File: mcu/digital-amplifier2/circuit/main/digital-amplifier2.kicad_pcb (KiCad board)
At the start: 2 copper layers, 94.5 x 100 mm, 166 parts, among them J1 I2C_oled, J10 Audio outA, J11 Audio outB, J12 Audio outC, J13 Audio outD, J2 encoder, J3 USB_C_Receptacle, J4 Conn_ARM_JTAG_SWD_20, J5 Barrel_Jack_Switch, J6 Conn_02x10_Odd_Even, J7 Conn_Coaxial, Q1 S8550, Q2 S8050, Q3 S8550, Q4 Q_NMOS_GDS, U1 DLT11H0, U12 TAS6424QDKQRQ1, U13 SJR-BTM331, U2 STM32F446RETx, U3 TPS54360DDA, U4 AMS1117-3.3, U5 LT3045xMSE-1, Y1 5032 8m

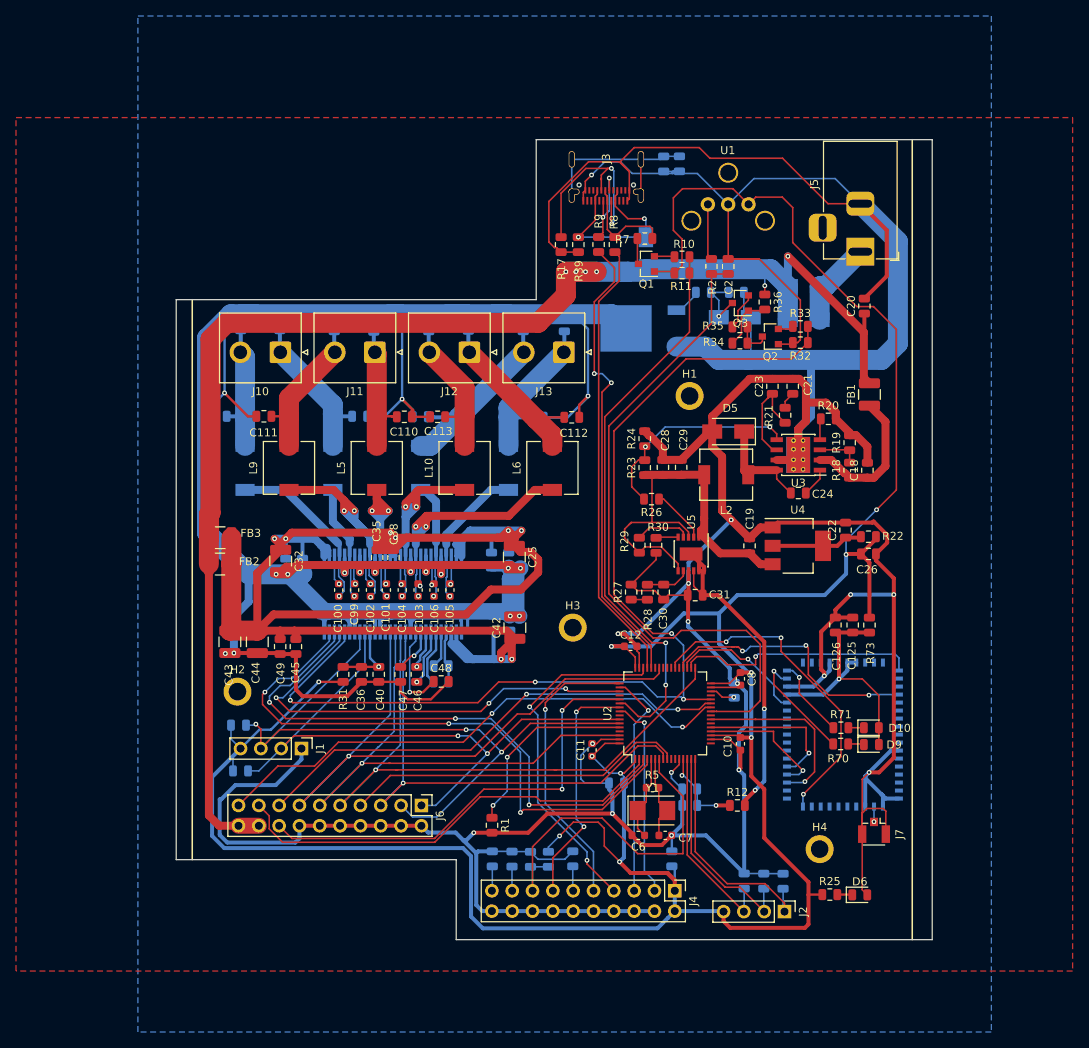
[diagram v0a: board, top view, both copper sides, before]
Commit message: headphone
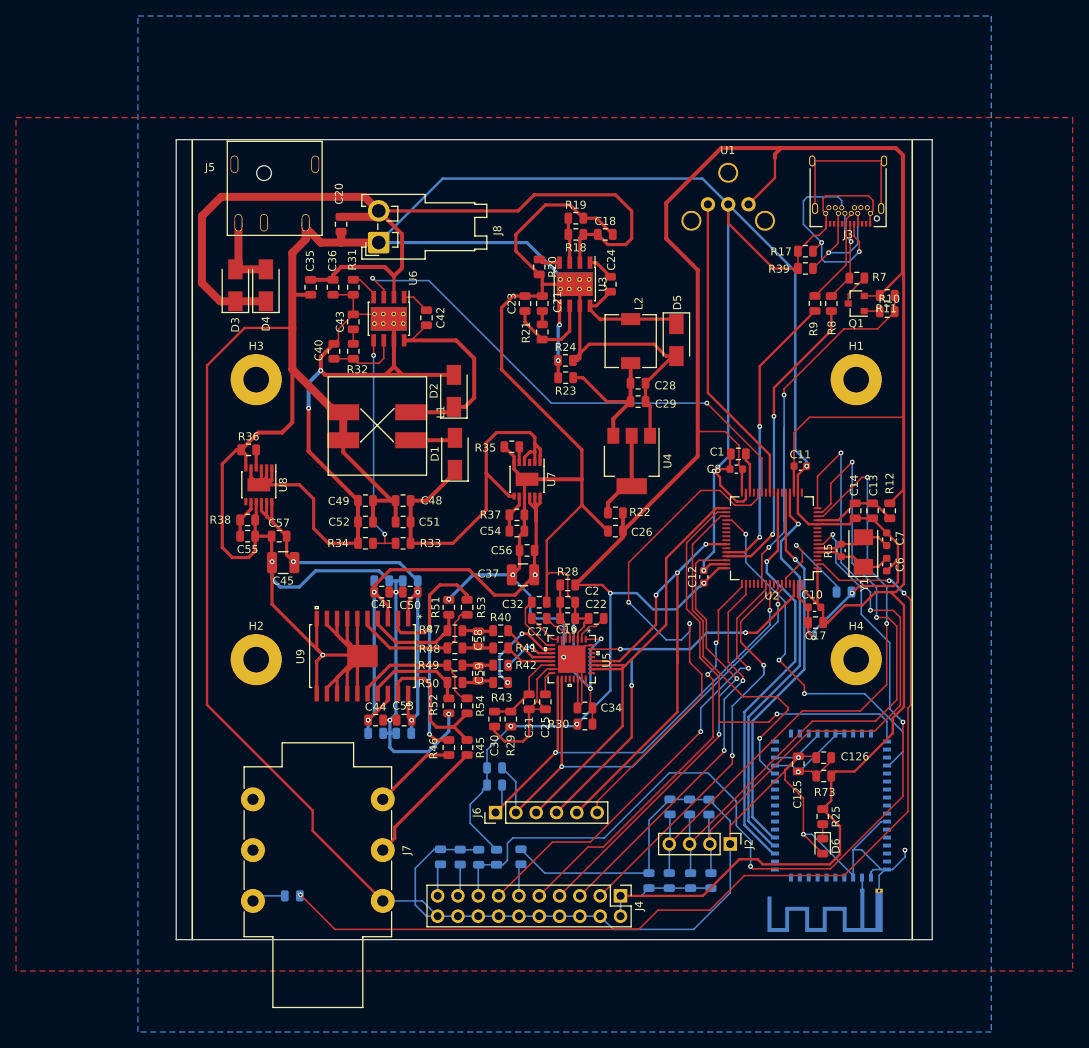
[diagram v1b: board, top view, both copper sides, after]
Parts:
- removed C100, C101, C102, C103, C104, C105, C106, C99: 1uf, Capacitor_SMD:C_0603_1608Metric
- removed C108, C109, C110, C111, C112, C113, C114, C115, C87, C88: 1uf, Capacitor_SMD:C_0805_2012Metric
- removed C117, C118, C119, C120, C121, C122, C123, C124: 1nf, Capacitor_SMD:C_0805_2012Metric
- removed C9: 1nF/1KV, Capacitor_SMD:C_0805_2012Metric
- removed D10, D9: LED, LED_SMD:LED_0805_2012Metric
- removed FB1, FB2, FB3: 300 ohm @100MHz 3.1A, Inductor_SMD:L_1210_3225Metric
- removed J1: I2C_oled, Connector_PinHeader_2.54mm:PinHeader_1x04_P2.54mm_Vertical
- removed J10: Audio outA, Connector_JST:JST_NV_B02P-NV_1x02_P5.00mm_Vertical
- removed J11: Audio outB, Connector_JST:JST_NV_B02P-NV_1x02_P5.00mm_Vertical
- removed J12: Audio outC, Connector_JST:JST_NV_B02P-NV_1x02_P5.00mm_Vertical
- removed J13: Audio outD, Connector_JST:JST_NV_B02P-NV_1x02_P5.00mm_Vertical
- removed L10, L11, L4, L5, L6, L7, L8, L9: 3.3uh, Inductor_SMD:L_6.3x6.3_H3
- removed Q2: S8050, Package_TO_SOT_SMD:SOT-23
- removed Q3: S8550, Package_TO_SOT_SMD:SOT-23
- removed Q4: Q_NMOS_GDS, Package_TO_SOT_SMD:TO-252-2
- removed R6: 1m, Resistor_SMD:R_0805_2012Metric
- removed R70, R71: 1k, Resistor_SMD:R_0805_2012Metric
- removed U12: TAS6424QDKQRQ1, ti:TAS6424QDKQRQ1
- added AE1: Antenna_Shield, RF_Antenna:Texas_SWRA117D_2.4GHz_Left, B.Cu at (135.8, 143.9)
- added C33: 100nf, Capacitor_SMD:C_0805_2012Metric, B.Cu at (98.9, 109.9)
- added C51: 22uf, Capacitor_SMD:C_0805_2012Metric, F.Cu at (78.4, 97.8)
- added C52: 22uf, Capacitor_SMD:C_0805_2012Metric, F.Cu at (73.7, 97.8)
- added C53: 100nf, Capacitor_SMD:C_0805_2012Metric, F.Cu at (78.5, 122.6)
- added C54: 4.7uf, Capacitor_SMD:C_0805_2012Metric, F.Cu at (92.6, 98.9)
- added C55: 4.7uf, Capacitor_SMD:C_0805_2012Metric, F.Cu at (58.9, 99.6)
- added C56: 10uf, Capacitor_SMD:C_0805_2012Metric, F.Cu at (93.9, 101.3)
- added C57: 10uf, Capacitor_SMD:C_0805_2012Metric, F.Cu at (62.9, 99.6)
- added C58: 100pf, Capacitor_SMD:C_0805_2012Metric, F.Cu at (87.8, 112.4)
- added C59: 100pf, Capacitor_SMD:C_0805_2012Metric, F.Cu at (87.8, 116.7)
- added J8: Conn_01x02, Connector_JST:JST_VH_S2P-VH_1x02_P3.96mm_Horizontal, F.Cu at (75.3, 62.9)
- added L1: 150uh, misc:MSD1278, F.Cu at (79.4, 84.1)
- added R40: 402Ω, Resistor_SMD:R_0805_2012Metric, F.Cu at (90.6, 111.4)
- added R41: 402Ω, Resistor_SMD:R_0805_2012Metric, F.Cu at (90.6, 113.5)
- added R42: 402Ω, Resistor_SMD:R_0805_2012Metric, F.Cu at (90.6, 115.7)
- added R43: 402Ω, Resistor_SMD:R_0805_2012Metric, F.Cu at (90.6, 117.9)
- added R44: 10k, Resistor_SMD:R_0805_2012Metric, B.Cu at (64.5, 144.5)
- added R45: 39.2Ω, Resistor_SMD:R_0805_2012Metric, F.Cu at (86.4, 126.0)
- added R46: 39.2Ω, Resistor_SMD:R_0805_2012Metric, F.Cu at (84.1, 126.0)
- added R47: 402Ω, Resistor_SMD:R_0805_2012Metric, F.Cu at (84.8, 111.4)
- added R48: 402Ω, Resistor_SMD:R_0805_2012Metric, F.Cu at (84.8, 113.5)
- added R49: 402Ω, Resistor_SMD:R_0805_2012Metric, F.Cu at (84.8, 115.7)
- added R50: 402Ω, Resistor_SMD:R_0805_2012Metric, F.Cu at (84.8, 117.9)
- added R51: 806Ω, Resistor_SMD:R_0805_2012Metric, F.Cu at (84.1, 108.5)
- added R52: 806Ω, Resistor_SMD:R_0805_2012Metric, F.Cu at (84.1, 120.8)
- added R53: 806Ω, Resistor_SMD:R_0805_2012Metric, F.Cu at (86.4, 108.5)
- added R54: 806Ω, Resistor_SMD:R_0805_2012Metric, F.Cu at (86.4, 120.8)
- added U6: TPS54360DDA, Package_SO:TI_SO-PowerPAD-8_ThermalVias, F.Cu at (76.6, 72.4)
- added U7: LT3045xMSE-1, Package_SO:MSOP-12-1EP_3x4mm_P0.65mm_EP1.65x2.85mm, F.Cu at (93.9, 92.5)
- added U8: LT3094xMSE, Package_SO:MSOP-12-1EP_3x4mm_P0.65mm_EP1.65x2.85mm, F.Cu at (60.3, 93.1)
- added U9: TPA6120A2DWP, ti:TPA6120A2DWP, F.Cu at (73.3, 114.6)
- C1, C13, C14, C17, C34, C41, C50, D1, D3, D4: moved to F.Cu
- C19, C31: value 10uf -> 100nf
- C2: value 10pf -> 10uf
- C22: value 100nf -> 0.1uf
- C25: value 100uf -> 1uf; footprint Capacitor_SMD:C_1210_3225Metric -> Capacitor_SMD:C_0805_2012Metric
- C27: value 10uf -> 2.2uf/25v; moved to F.Cu
- C30: value 4.7uf -> 10uf
- C32: value 100uf -> 2.2uF/25V; footprint Capacitor_SMD:C_1210_3225Metric -> Capacitor_SMD:C_0805_2012Metric
- C36: value 10uf -> 1uf
- C37: value 100nf -> 100uf; footprint Capacitor_SMD:C_0805_2012Metric -> Capacitor_SMD:C_1210_3225Metric; moved to F.Cu
- C38: value 100nf -> 10uf; moved to B.Cu
- C40: value 100nf -> 750pf
- C42: value 100uf -> 0.1uf; footprint Capacitor_SMD:C_1210_3225Metric -> Capacitor_SMD:C_0805_2012Metric
- C43: value 100uf -> 5.1nf; footprint Capacitor_SMD:C_1210_3225Metric -> Capacitor_SMD:C_0805_2012Metric
- C44: value 100uf -> 100nf; footprint Capacitor_SMD:C_1210_3225Metric -> Capacitor_SMD:C_0805_2012Metric
- C45: value 100nf -> 100uf; footprint Capacitor_SMD:C_0805_2012Metric -> Capacitor_SMD:C_1210_3225Metric
- C46: value 1uf -> 10uf; moved to B.Cu
- C47: value 2.2uf -> 10uf; moved to B.Cu
- C48: value 2.2uf -> 22uf
- C49: value 1uf -> 22uf
- D2: value 10v -> 60v 3A; moved to F.Cu
- H1: value m2_1 -> m3; footprint MountingHole:MountingHole_2.2mm_M2_ISO7380_Pad -> MountingHole:MountingHole_3.2mm_M3_Pad
- H2: value m2_2 -> m3; footprint MountingHole:MountingHole_2.2mm_M2_ISO7380_Pad -> MountingHole:MountingHole_3.2mm_M3_Pad
- H3: value m2_3 -> m3; footprint MountingHole:MountingHole_2.2mm_M2_ISO7380_Pad -> MountingHole:MountingHole_3.2mm_M3_Pad
- H4: value m2_4 -> m3; footprint MountingHole:MountingHole_2.2mm_M2_ISO7380_Pad -> MountingHole:MountingHole_3.2mm_M3_Pad
- J3: footprint connector:usb_c_24p_smd -> Connector_USB:USB_C_Receptacle_Amphenol_12401548E4-2A
- J5: footprint Connector_BarrelJack:BarrelJack_Horizontal -> connector:DC-044A_5.5-2.1
- J6: value Conn_02x10_Odd_Even -> Conn_01x06; footprint Connector_PinHeader_2.54mm:PinHeader_2x10_P2.54mm_Vertical -> Connector_PinHeader_2.54mm:PinHeader_1x06_P2.54mm_Vertical
- J7: value Conn_Coaxial -> AudioJack3_Switch; footprint Connector_Coaxial:U.FL_Hirose_U.FL-R-SMT-1_Vertical -> Connector_Audio:Jack_6.35mm_Neutrik_NMJ6HFD2_Horizontal
- Q1: value S8550 -> s8550
- R1: moved to B.Cu
- R2: value 49.9Ω -> 9.53k; moved to B.Cu
- R26: value test point -> 9.53k; moved to B.Cu
- R27: value 33.2k -> 9.53k; moved to B.Cu
- R29: value 200k -> 0Ω
- R31: value 0Ω -> 49.9k
- R32: value 10k -> 15.4k
- R33: value 10k -> 215k
- R34: value 10k -> 12.1k
- R35: value 10k -> 200k
- R36: value 10kΩ -> 200k
- R37, R38: value 10k -> 150k; moved to F.Cu
- U5: value LT3045xMSE-1 -> PCM5242; footprint Package_SO:MSOP-12-1EP_3x4mm_P0.65mm_EP1.65x2.85mm -> ti:PCM5242RHBR
- moved J5 79.0 mm to (57.3, 53.1), turned to 0 degrees
- moved R2 77.0 mm to (111.6, 142.6)
- moved D3 71.2 mm to (57.4, 68.2), turned to 90 degrees
- moved D4 67.3 mm to (61.2, 68.2), turned to 90 degrees
- moved R36 67.1 mm to (59.1, 88.8), turned to 0 degrees
- moved C20 66.2 mm to (70.6, 60.6), turned to 270 degrees
- moved R38 63.7 mm to (58.9, 97.5), turned to 180 degrees
- moved J7 61.5 mm to (75.8, 132.5)
- moved R33 56.6 mm to (78.4, 100.5), turned to 180 degrees
- moved R32 55.9 mm to (72.1, 76.5), turned to 90 degrees
- moved R34 53.1 mm to (73.7, 100.5), turned to 180 degrees
- moved R1 52.8 mm to (133.5, 106.6), turned to 0 degrees
- moved H3 50.3 mm to (60.0, 80.0)
- moved C36 48.5 mm to (69.6, 68.5)
- moved R31 48.4 mm to (72.1, 68.5)
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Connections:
- C18 pad 1: Net-(C18-Pad1) -> VCC
- C19 pad 1: VDD -> /Sheet6035C8EF/CPVDD
- C2 pad 1: /stm32/SPDIF_RX -> /Sheet6035C8EF/CPVDD
- C25 pad 1: /TAS6424/vcc_x -> GND
- C25 pad 2: /TAS6424/gnd_x -> Net-(C25-Pad2)
- C27 pad 1: /TAS6424/vcc_x -> Net-(C27-Pad1)
- C27 pad 2: /TAS6424/gnd_x -> Net-(C27-Pad2)
- C30 pad 1: Net-(C30-Pad1) -> /Sheet6035C8EF/AVDD
- C31 pad 1: +3.3VA -> /Sheet6035C8EF/AVDD
- C32 pad 1: /TAS6424/vcc_x -> Net-(C32-Pad1)
- C32 pad 2: /TAS6424/gnd_x -> GND
- C34 pad 1: /TAS6424/vcc_x -> /Sheet6035C8EF/DVDD
- C34 pad 2: /TAS6424/gnd_x -> GND
- C35 pad 1: /TAS6424/vcc_x -> VCC
- C35 pad 2: /TAS6424/gnd_x -> GND
- C36 pad 1: /TAS6424/tas6424_power/vdd_33 -> VCC
- C36 pad 2: /TAS6424/gnd_x -> Net-(C36-Pad2)
- C37 pad 1: /TAS6424/vcc_x -> +15V
- C37 pad 2: /TAS6424/gnd_x -> GND
- C38 pad 1: /TAS6424/vcc_x -> +15V
- C38 pad 2: /TAS6424/gnd_x -> GND
- C39 pad 1: /TAS6424/vcc_x -> +15V
- C39 pad 2: /TAS6424/gnd_x -> GND
- C40 pad 1: /TAS6424/tas6424_power/vdd_33 -> Net-(C40-Pad1)
- C40 pad 2: /TAS6424/gnd_x -> Net-(C36-Pad2)
- C41 pad 1: /TAS6424/vcc_x -> +15V
- C41 pad 2: /TAS6424/gnd_x -> GND
- C42 pad 1: /TAS6424/vcc_x -> Net-(C42-Pad1)
- C42 pad 2: /TAS6424/gnd_x -> Net-(C42-Pad2)
- C43 pad 1: /TAS6424/vcc_x -> Net-(C43-Pad1)
- C43 pad 2: /TAS6424/gnd_x -> Net-(C36-Pad2)
- C44 pad 1: /TAS6424/vcc_x -> +15V
- C44 pad 2: /TAS6424/gnd_x -> GND
- C45 pad 1: /TAS6424/vcc_x -> -15V
- C45 pad 2: /TAS6424/gnd_x -> GND
- C46 pad 1: Net-(C46-Pad1) -> -15V
- C46 pad 2: Net-(C46-Pad2) -> GND
- C47 pad 1: Net-(C47-Pad1) -> -15V
- C47 pad 2: /TAS6424/gnd_x -> GND
- C48 pad 2: /TAS6424/gnd_x -> GND
- C49 pad 1: /TAS6424/vcc_x -> GND
- C49 pad 2: /TAS6424/gnd_x -> Net-(C36-Pad2)
- C50 pad 1: /TAS6424/vcc_x -> -15V
- C50 pad 2: /TAS6424/gnd_x -> GND
- D1 pad 1: VCC -> Net-(C48-Pad1)
- D2 pad 1: Net-(D2-Pad1) -> Net-(C42-Pad1)
- D2 pad 2: GND -> Net-(C36-Pad2)
- H1 pad 1: (no net) -> Net-(H1-Pad1)
- H2 pad 1: (no net) -> Net-(H2-Pad1)
- H3 pad 1: (no net) -> Net-(H3-Pad1)
- H4 pad 1: (no net) -> Net-(H4-Pad1)
- J2 pad 1: /stm32/encoder_b -> GND
- J2 pad 2: /stm32/encoder_a -> /stm32/encoder_b
- J2 pad 3: /stm32/encoder_sw -> /stm32/encoder_a
- J2 pad 4: +3V3 -> /stm32/encoder_sw
- J3 pad A4: Net-(D1-Pad2) -> Net-(J3-PadA4)
- J3 pad A9: Net-(D1-Pad2) -> Net-(J3-PadA4)
- J3 pad B4: Net-(D1-Pad2) -> Net-(J3-PadA4)
- J3 pad B9: Net-(D1-Pad2) -> Net-(J3-PadA4)
- J6 pad 2: GND -> /SDA
- J6 pad 3: /SDA -> /SAI1_B_CLK
- J6 pad 4: GND -> /SAI1_B_FS
- J6 pad 5: /SAI1_B_MCK -> /SAI1_B_SD
- J6 pad 6: GND -> /tas6424_en
- Q1 pad 1: +3V3 -> Net-(Q1-Pad1)
- Q1 pad 2: Net-(Q1-Pad2) -> +3V3
- R10 pad 2: Net-(Q1-Pad2) -> Net-(Q1-Pad1)
- R12 pad 2: +3.3VA -> +3V3
- R18 pad 1: Net-(C18-Pad1) -> VCC
- R2 pad 1: /stm32/SPDIF_RX -> +3V3
- R2 pad 2: Net-(R2-Pad2) -> /stm32/encoder_sw
- R22 pad 2: Net-(C22-Pad1) -> Net-(R22-Pad2)
- R26 pad 1: Net-(R26-Pad1) -> +3V3
- R26 pad 2: Net-(R23-Pad2) -> /stm32/encoder_a
- R27 pad 1: Net-(R27-Pad1) -> +3V3
- R27 pad 2: GND -> /stm32/encoder_b
- R28 pad 1: Net-(C30-Pad1) -> /Sheet6035C8EF/CPVDD
- R28 pad 2: Net-(R27-Pad1) -> +3V3
- R29 pad 1: Net-(R29-Pad1) -> /Sheet6035C8EF/AVDD
- R29 pad 2: VDD -> +3V3
- R30 pad 1: GND -> /Sheet6035C8EF/DVDD
- R30 pad 2: Net-(R30-Pad2) -> +3V3
- R31 pad 1: /TAS6424/tas6424_power/vdd_33 -> Net-(R31-Pad1)
- R31 pad 2: +3V3 -> Net-(C36-Pad2)
- R32 pad 1: /tas6424_en -> Net-(C40-Pad1)
- R32 pad 2: GND -> Net-(C43-Pad1)
- R33 pad 1: Net-(Q2-Pad2) -> Net-(C48-Pad1)
- R33 pad 2: /tas6424_en -> Net-(R33-Pad2)
- R34 pad 1: Net-(Q3-Pad1) -> Net-(R33-Pad2)
- R34 pad 2: Net-(Q2-Pad3) -> Net-(C36-Pad2)
- R35 pad 2: Net-(Q2-Pad3) -> GND
- R36 pad 1: VCC -> GND
- R36 pad 2: Net-(Q3-Pad1) -> Net-(R36-Pad2)
- R37 pad 1: Net-(D2-Pad1) -> Net-(C54-Pad1)
- R38 pad 1: Net-(Q4-Pad1) -> GND
- R38 pad 2: Net-(D2-Pad1) -> Net-(C55-Pad2)
- R39 pad 1: Net-(D1-Pad2) -> Net-(J3-PadA4)
- U1 pad 1: Net-(R2-Pad2) -> /stm32/SPDIF_RX
- U13 pad 46: Net-(J7-Pad1) -> Net-(AE1-Pad1)
- U13 pad 54: /BT_spdif -> Net-(U13-Pad54)
- U2 pad 26: /headphone_mute -> Net-(U2-Pad26)
- U2 pad 3: /tas6424_fault -> Net-(U2-Pad3)
- U2 pad 38: /BT_spdif -> Net-(U2-Pad38)
- U2 pad 4: /tas6424_warn -> Net-(U2-Pad4)
- U2 pad 51: /tas6424_mute -> Net-(U2-Pad51)
- U2 pad 53: /headphone_irq -> Net-(U2-Pad53)
- U2 pad 8: /SAI1_B_MCK -> Net-(U2-Pad8)
- U2 pad 9: /SAI1_A_SD -> Net-(U2-Pad9)
- U3 pad 2: Net-(C18-Pad1) -> VCC
- U4 pad 2: Net-(C22-Pad1) -> Net-(R22-Pad2)
- U5 pad 1: VDD -> /Sheet6035C8EF/DVDD
- U5 pad 10: +3.3VA -> /Sheet6035C8EF/OUTLP
- U5 pad 11: +3.3VA -> /Sheet6035C8EF/OUTLN
- U5 pad 12: +3.3VA -> /Sheet6035C8EF/OUTRP
- U5 pad 13: +3.3VA -> /Sheet6035C8EF/OUTRN
- U5 pad 2: VDD -> Net-(C22-Pad1)
- U5 pad 3: Net-(R26-Pad1) -> GND
- U5 pad 4: VDD -> /Sheet6035C8EF/DVDD
- U5 pad 5: Net-(R29-Pad1) -> /Sheet6035C8EF/CPVDD
- U5 pad 6: Net-(R30-Pad2) -> Net-(C27-Pad2)
- U5 pad 7: VDD -> GND
- U5 pad 8: Net-(C30-Pad1) -> Net-(C27-Pad1)
- U5 pad 9: GND -> Net-(C32-Pad1)
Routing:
- net /TAS6424/gnd_x: track 463.3 -> 0.00 mm, vias 17 -> 0
- net GND: track 676.5 -> 1003.8 mm
- net /TAS6424/vcc_x: track 242.0 -> 0.00 mm, vias 8 -> 0
- net Net-(C36-Pad2): track 0.00 -> 106.3 mm, vias 0 -> 2
- net /tas6424_warn: track 74.8 -> 0.00 mm, vias 3 -> 0
- net /tas6424_fault: track 71.2 -> 0.00 mm, vias 3 -> 0
- net /headphone_in: track 55.6 -> 123.9 mm, vias 0 -> 3
- net /tas6424_en: track 135.6 -> 67.3 mm, vias 4 -> 2
- net /stm32/NRST: track 46.0 -> 114.2 mm, vias 0 -> 3
- net +15V: track 0.00 -> 67.7 mm, vias 0 -> 3
- net /headphone_mute: track 67.0 -> 0.00 mm, vias 2 -> 0
- net VCC: track 183.2 -> 117.8 mm, vias 6 -> 0
- net /SAI1_B_MCK: track 62.4 -> 0.00 mm, vias 1 -> 0
- net /tas6424_mute: track 57.0 -> 0.00 mm, vias 3 -> 0
- net -15V: track 0.00 -> 56.9 mm, vias 0 -> 3
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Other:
- outline, holes or cut-outs redrawn
- net class Default: clearance 0.15 -> 0.2
- rule trace_clearance: 0.15 -> 0.2

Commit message: v3
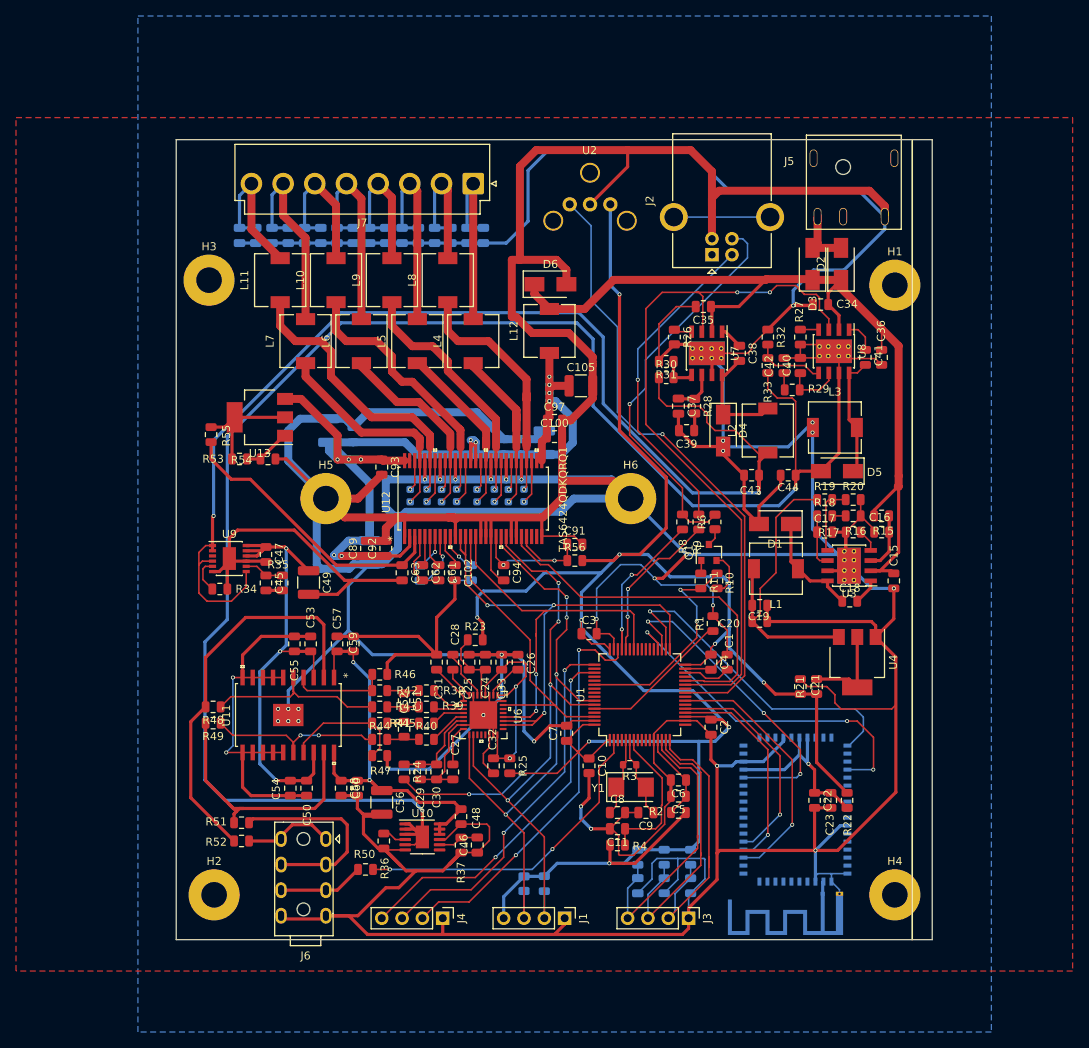
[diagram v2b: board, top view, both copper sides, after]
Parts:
- removed C125: 22uf, Capacitor_SMD:C_0805_2012Metric
- removed C126: 10uf, Capacitor_SMD:C_0805_2012Metric
- removed the C22 at (102.5, 109.9)
- removed the C25 at (96.1, 120.3)
- removed the C27 at (95.4, 109.9)
- removed the C32 at (95.4, 107.8)
- removed the C42 at (81.3, 72.3)
- removed the C43 at (72.1, 72.8)
- removed the C44 at (74.9, 122.6)
- removed the C47 at (78.4, 124.2)
- removed the C53 at (78.5, 122.6)
- removed the C58 at (87.8, 112.4)
- removed J8: Conn_01x02, Connector_JST:JST_VH_S2P-VH_1x02_P3.96mm_Horizontal
- removed the R27 at (116.8, 142.6)
- removed the R40 at (90.6, 111.4)
- removed the R41 at (90.6, 113.5)
- removed the R42 at (90.6, 115.7)
- removed the R43 at (90.6, 117.9)
- removed the R49 at (84.8, 115.7)
- removed the R50 at (84.8, 117.9)
- removed R73: 0Ω, Resistor_SMD:R_0805_2012Metric
- added C100: 100nf, Capacitor_SMD:C_0805_2012Metric, F.Cu at (97.3, 87.1)
- added C101: 1uf, Capacitor_SMD:C_0805_2012Metric, B.Cu at (80.5, 104.2)
- added C102: 2.2uf, Capacitor_SMD:C_0805_2012Metric, F.Cu at (84.8, 104.1)
- added C103: 2.2uf, Capacitor_SMD:C_0805_2012Metric, B.Cu at (86.9, 104.1)
- added C105: 100uf, Capacitor_SMD:C_1210_3225Metric, F.Cu at (100.6, 80.8)
- added C24: 10uf, Capacitor_SMD:C_0805_2012Metric, F.Cu at (88.6, 115.3)
- added C26: 0.1uf, Capacitor_SMD:C_0805_2012Metric, F.Cu at (92.7, 115.3)
- added C29: 10uf, Capacitor_SMD:C_0805_2012Metric, F.Cu at (80.5, 129.0)
- added C35: 2.2uf, Capacitor_SMD:C_0805_2012Metric, F.Cu at (115.9, 70.9)
- added C38: 100nf, Capacitor_SMD:C_0805_2012Metric, F.Cu at (120.4, 76.7)
- added C39: 1.2nf, Capacitor_SMD:C_0805_2012Metric, F.Cu at (113.8, 86.4)
- added C40: 1.3pf, Capacitor_SMD:C_0805_2012Metric, F.Cu at (128.0, 78.2)
- added C45: 4.7uf, Capacitor_SMD:C_0805_2012Metric, F.Cu at (61.2, 105.4)
- added C48: 10uf, Capacitor_SMD:C_0805_2012Metric, F.Cu at (85.6, 134.6)
- added C54: 100nf, Capacitor_SMD:C_0805_2012Metric, F.Cu at (64.3, 131.1)
- added C60: 100nf, Capacitor_SMD:C_0805_2012Metric, F.Cu at (72.6, 131.1)
- added C61: 1uf, Capacitor_SMD:C_0805_2012Metric, F.Cu at (82.8, 104.1)
- added C62: 1uf, Capacitor_SMD:C_0805_2012Metric, F.Cu at (80.8, 104.1)
- added C63: 10uf, Capacitor_SMD:C_0805_2012Metric, F.Cu at (78.2, 104.1)
- added C64: 1uf, Capacitor_SMD:C_0603_1608Metric, B.Cu at (91.5, 94.5)
- added C65: 1uf, Capacitor_SMD:C_0603_1608Metric, B.Cu at (93.5, 94.5)
- added C66: 1uf, Capacitor_SMD:C_0603_1608Metric, B.Cu at (87.6, 94.5)
- added C67: 1uf, Capacitor_SMD:C_0603_1608Metric, B.Cu at (89.8, 94.5)
- added C68: 1uf, Capacitor_SMD:C_0603_1608Metric, B.Cu at (83.2, 94.5)
- added C69: 1uf, Capacitor_SMD:C_0603_1608Metric, B.Cu at (85.1, 94.5)
- added C70: 1uf, Capacitor_SMD:C_0603_1608Metric, B.Cu at (79.2, 94.5)
- added C71: 1uf, Capacitor_SMD:C_0603_1608Metric, B.Cu at (81.4, 94.5)
- added C72: 1uf, Capacitor_SMD:C_0805_2012Metric, B.Cu at (86.4, 62.0)
- added C73: 1uf, Capacitor_SMD:C_0805_2012Metric, B.Cu at (82.3, 62.0)
- added C74: 1uf, Capacitor_SMD:C_0805_2012Metric, B.Cu at (78.2, 62.0)
- added C75: 1uf, Capacitor_SMD:C_0805_2012Metric, B.Cu at (74.2, 62.0)
- added C76: 1uf, Capacitor_SMD:C_0805_2012Metric, B.Cu at (70.1, 62.0)
- added C77: 1uf, Capacitor_SMD:C_0805_2012Metric, B.Cu at (66.0, 62.0)
- added C78: 1uf, Capacitor_SMD:C_0805_2012Metric, B.Cu at (62.0, 62.0)
- added C79: 1uf, Capacitor_SMD:C_0805_2012Metric, B.Cu at (57.9, 62.0)
- added C80: 1nf, Capacitor_SMD:C_0805_2012Metric, B.Cu at (88.4, 62.0)
- added C81: 1nf, Capacitor_SMD:C_0805_2012Metric, B.Cu at (84.3, 62.0)
- added C82: 1nf, Capacitor_SMD:C_0805_2012Metric, B.Cu at (80.3, 62.0)
- added C83: 1nf, Capacitor_SMD:C_0805_2012Metric, B.Cu at (76.2, 62.0)
- added C84: 1nf, Capacitor_SMD:C_0805_2012Metric, B.Cu at (72.1, 62.0)
- added C85: 1nf, Capacitor_SMD:C_0805_2012Metric, B.Cu at (68.1, 62.0)
- added C86: 1nf, Capacitor_SMD:C_0805_2012Metric, B.Cu at (64.0, 62.0)
- added C87: 1nf, Capacitor_SMD:C_0805_2012Metric, B.Cu at (59.9, 62.0)
- added C88: 100uf, Capacitor_SMD:C_1210_3225Metric, B.Cu at (74.2, 101.6)
- added C89: 10uf, Capacitor_SMD:C_0805_2012Metric, F.Cu at (73.8, 101.1)
- added C9: 12pf, Capacitor_SMD:C_0805_2012Metric, F.Cu at (108.7, 134.1)
- added C90: 10uf, Capacitor_SMD:C_0805_2012Metric, B.Cu at (72.1, 86.9)
- added C91: 10uf, Capacitor_SMD:C_0805_2012Metric, F.Cu at (99.8, 100.6)
- added C92: 100nf, Capacitor_SMD:C_0805_2012Metric, F.Cu at (76.2, 101.1)
- added C93: 100nf, Capacitor_SMD:C_0805_2012Metric, F.Cu at (75.7, 90.9)
- added C94: 100nf, Capacitor_SMD:C_0805_2012Metric, F.Cu at (90.9, 104.1)
- added C95: 100uf, Capacitor_SMD:C_1210_3225Metric, B.Cu at (96.0, 87.9)
- added C96: 100uf, Capacitor_SMD:C_1210_3225Metric, B.Cu at (69.1, 86.4)
- added C97: 10uf, Capacitor_SMD:C_0805_2012Metric, F.Cu at (97.3, 85.1)
- added C98: 10uf, Capacitor_SMD:C_0805_2012Metric, B.Cu at (93.0, 88.4)
- added C99: 100nf, Capacitor_SMD:C_0805_2012Metric, B.Cu at (90.9, 88.4)
- added H5: m3, MountingHole:MountingHole_3.2mm_M3_Pad, F.Cu at (68.7, 94.9)
- added H6: m3, MountingHole:MountingHole_3.2mm_M3_Pad, F.Cu at (106.8, 94.9)
- added J1: i2c, Connector_PinHeader_2.54mm:PinHeader_1x04_P2.54mm_Vertical, F.Cu at (98.6, 147.3)
- added L10: 3.3uh, Inductor_SMD:L_6.3x6.3_H3, F.Cu at (70.0, 67.6)
- added L11: 3.3uh, Inductor_SMD:L_6.3x6.3_H3, F.Cu at (63.0, 67.6)
- added L12: 4.7uh, Inductor_SMD:L_6.3x6.3_H3, F.Cu at (96.6, 73.9)
- added L3: 22uh, Inductor_SMD:L_6.3x6.3_H3, F.Cu at (132.3, 86.0)
- added L4: 3.3uh, Inductor_SMD:L_6.3x6.3_H3, F.Cu at (87.1, 75.2)
- added L5: 3.3uh, Inductor_SMD:L_6.3x6.3_H3, F.Cu at (80.1, 75.2)
- added L6: 3.3uh, Inductor_SMD:L_6.3x6.3_H3, F.Cu at (73.2, 75.2)
- added L7: 3.3uh, Inductor_SMD:L_6.3x6.3_H3, F.Cu at (66.2, 75.2)
- added L8: 3.3uh, Inductor_SMD:L_6.3x6.3_H3, F.Cu at (83.9, 67.6)
- added L9: 3.3uh, Inductor_SMD:L_6.3x6.3_H3, F.Cu at (77.0, 67.6)
- added R26: 121k, Resistor_SMD:R_0805_2012Metric, F.Cu at (112.3, 74.7)
- added R28: 68.1k, Resistor_SMD:R_0805_2012Metric, F.Cu at (114.8, 83.3)
- added R30: 215k, Resistor_SMD:R_0805_2012Metric, F.Cu at (111.3, 79.8)
- added R31: 12.1k, Resistor_SMD:R_0805_2012Metric, F.Cu at (111.3, 77.7)
- added R33: 12.1k, Resistor_SMD:R_0805_2012Metric, F.Cu at (124.0, 78.2)
- added R45: 402Ω, Resistor_SMD:R_0805_2012Metric, F.Cu at (75.4, 122.9)
- added R46: 806Ω, Resistor_SMD:R_0805_2012Metric, F.Cu at (75.4, 116.8)
- added R55: 0Ω, Resistor_SMD:R_0805_2012Metric, F.Cu at (54.4, 86.9)
- added R56: 0Ω, Resistor_SMD:R_0805_2012Metric, F.Cu at (99.8, 102.6)
- added R6: 1.5k, Resistor_SMD:R_0805_2012Metric, F.Cu at (117.3, 97.8)
- added U11: TPA6120A2DWP, ti:TPA6120A2DWP, F.Cu at (64.0, 121.9)
- added U12: TAS6424QDKQRQ1, ti:TAS6424QDKQRQ1, F.Cu at (87.1, 94.9)
- added U7: TPS54360DDA, Package_SO:TI_SO-PowerPAD-8_ThermalVias, F.Cu at (116.3, 76.7)
- C10: value 100nf/10v -> 100nf; footprint Capacitor_SMD:C_0603_1608Metric -> Resistor_SMD:R_0805_2012Metric
- C11: value 100nf/10v -> 100nf; footprint Capacitor_SMD:C_0603_1608Metric -> Capacitor_SMD:C_0805_2012Metric
- C12: value 100nf/10v -> 100nf; footprint Capacitor_SMD:C_0603_1608Metric -> Capacitor_SMD:C_0805_2012Metric; moved to B.Cu
- C13: value 10uf -> 100nf; moved to B.Cu
- C14: moved to B.Cu
- C15: value 100nf -> 4.7uf; moved to F.Cu
- C16: value 100nf -> 6.8nf; moved to F.Cu
- C17: value 100nf -> 39pf; footprint Resistor_SMD:R_0805_2012Metric -> Capacitor_SMD:C_0805_2012Metric
- C18: value 4.7uf -> 100nf
- C19: value 100nf -> 47uf
- C2: value 10uf -> 100nf/10v
- C20: value 4.7uf -> 47uf
- C21: value 6.8nf -> 10uf
- C22: renamed from C23; value 39pf -> 22uf
- C23: renamed from C24; value 100nf -> 10uf
- C25: renamed from C26; value 10uf -> 100nf
- C27: renamed from C28; value 47uf -> 1uf
- C28: renamed from C29; value 47uf -> 2.2uf/25v
- C3, C4: value 100nf -> 100nf/10v; moved to F.Cu
- C30: value 10uf -> 100nf
- C31: value 100nf -> 2.2uF/25V
- C32: renamed from C33; moved to F.Cu
- C34: renamed from C35; value 10uf -> 2.2uf
- C36: value 1uf -> 2.2uf
- C37: value 100uf -> 1.3pf; footprint Capacitor_SMD:C_1210_3225Metric -> Capacitor_SMD:C_0805_2012Metric
- C41: renamed from C38; value 10uf -> 100nf; moved to F.Cu
- C42: renamed from C39; value 10uf -> 1.2nf; moved to F.Cu
- C43: renamed from C40; value 750pf -> 22uf
- C44: renamed from C41; value 100nf -> 22uf
- C46: renamed from C45; value 100uf -> 4.7uf; footprint Capacitor_SMD:C_1210_3225Metric -> Capacitor_SMD:C_0805_2012Metric
- C47: renamed from C46; moved to F.Cu
- C49: renamed from C48; value 22uf -> 100uf; footprint Capacitor_SMD:C_0805_2012Metric -> Capacitor_SMD:C_1210_3225Metric
- C5: value 100nf -> 10uf; moved to F.Cu
- C50: renamed from C49; value 22uf -> 10uf
- C51: renamed from C50; value 100nf -> 1nf
- C52: renamed from C51; value 22uf -> 1nf
- C53: renamed from C52; value 22uf -> 10uf
- C55: renamed from C54; value 4.7uf -> 100nf
- C56: renamed from C55; value 4.7uf -> 100uf; footprint Capacitor_SMD:C_0805_2012Metric -> Capacitor_SMD:C_1210_3225Metric
- C59: value 100pf -> 100nf
- C6: value 12pf -> 100nf; footprint Capacitor_SMD:C_0603_1608Metric -> Capacitor_SMD:C_0805_2012Metric
- C7: value 12pf -> 100nf/10v; footprint Capacitor_SMD:C_0603_1608Metric -> Capacitor_SMD:C_0805_2012Metric
- C8: value 100nf/10v -> 12pf; footprint Capacitor_SMD:C_0603_1608Metric -> Capacitor_SMD:C_0805_2012Metric
- D1: value 60v 3A -> B560C
- D2: value 60v 3A -> 40v 5A
- D4: value 40v 5A -> 60v/3A
- D5: value B560C -> 60v 3A
- D6: value 0805 -> D; footprint LED_SMD:LED_0805_2012Metric -> Diode_SMD:D_SMA
- J2: value encoder -> USB_B; footprint Connector_PinHeader_2.54mm:PinHeader_1x04_P2.54mm_Vertical -> Connector_USB:USB_B_OST_USB-B1HSxx_Horizontal
- J3: value USB_C_Receptacle -> encoder; footprint Connector_USB:USB_C_Receptacle_Amphenol_12401548E4-2A -> Connector_PinHeader_2.54mm:PinHeader_1x04_P2.54mm_Vertical
- J4: value Conn_ARM_JTAG_SWD_20 -> swd; footprint Connector_PinHeader_2.54mm:PinHeader_2x10_P2.54mm_Vertical -> Connector_PinHeader_2.54mm:PinHeader_1x04_P2.54mm_Vertical
- J6: value Conn_01x06 -> AudioJack4; footprint Connector_PinHeader_2.54mm:PinHeader_1x06_P2.54mm_Vertical -> connector:Jack_3.5mm_4pin
- J7: value AudioJack3_Switch -> Conn_01x08; footprint Connector_Audio:Jack_6.35mm_Neutrik_NMJ6HFD2_Horizontal -> Connector_JST:JST_VH_B8P-VH-B_1x08_P3.96mm_Vertical
- L1: value 150uh -> 8.2uh; footprint misc:MSD1278 -> Inductor_SMD:L_6.3x6.3_H3
- L2: value 8.2uh -> 22uh
- R1: moved to F.Cu
- R10: value 5.1k -> 22k
- R11: value 22k -> 5.1k
- R12: value 0Ω -> 9.53k; moved to B.Cu
- R13: value 22k -> 9.53k
- R14: value 10k -> 9.53k
- R15: value 10k -> 523k; moved to F.Cu
- R16: value 10k -> 84.5k; moved to F.Cu
- R17: value 5.1k -> 162k
- R18: value 523k -> 13k
- R19: value 84.5k -> 53.6k
- R2: value 9.53k -> 0Ω; moved to F.Cu
- R20: value 162k -> 10.2k
- R21: value 13k -> 0Ω
- R23: value 53.6k -> 0Ω
- R24: value 10.2k -> 0Ω
- R25: value 20k -> 0Ω
- R27: renamed from R26; value 9.53k -> 121k; moved to F.Cu
- R29: value 0Ω -> 68.1k
- R3: value 4.7k -> 1mΩ; footprint Resistor_SMD:R_0805_2012Metric -> Resistor_SMD:R_0603_1608Metric; moved to F.Cu
- R32: renamed from R28; value 0Ω -> 215k
- R34: renamed from R30; value 0Ω -> 200k
- R35: renamed from R32; value 15.4k -> 150k
- R36: renamed from R31; value 49.9k -> 200k
- R37: renamed from R33; value 215k -> 150k
- R38: renamed from R34; value 12.1k -> 402Ω
- R39: renamed from R35; value 200k -> 402Ω
- R4: value 4.7k -> 9.53k; moved to F.Cu
- R40: renamed from R36; value 200k -> 402Ω
- R41: renamed from R37; value 150k -> 402Ω
- R42: renamed from R38; value 150k -> 402Ω
- R43: renamed from R39; value 1m -> 402Ω
- R44: value 10k -> 402Ω; moved to F.Cu
- R47, R48: value 402Ω -> 806Ω
- R49: renamed from R45; value 39.2Ω -> 806Ω
- R5: value 1mΩ -> 4.7k; footprint Resistor_SMD:R_0603_1608Metric -> Resistor_SMD:R_0805_2012Metric; moved to B.Cu
- R50: renamed from R46; value 39.2Ω -> 9.53k
- R51, R52: value 806Ω -> 39.2Ω
- R53: value 806Ω -> 9.53k
- R54: value 806Ω -> 1k
- R7: value 1.5k -> 4.7k; moved to B.Cu
- U1: value DLT11H0 -> STM32F446RETx; footprint connector:spdif-DLT11H0 -> Package_QFP:LQFP-64_10x10mm_P0.5mm
- U10: renamed from U9; value TPA6120A2DWP -> LT3094xMSE; footprint ti:TPA6120A2DWP -> Package_SO:MSOP-12-1EP_3x4mm_P0.65mm_EP1.65x2.85mm
- U13: value SJR-BTM331 -> LM317_SOT-223; footprint misc:SJR-BTM331 -> Package_TO_SOT_SMD:SOT-223-3_TabPin2; moved to F.Cu
- U2: value STM32F446RETx -> DLT11H0; footprint Package_QFP:LQFP-64_10x10mm_P0.5mm -> connector:spdif-DLT11H0
- U5: value PCM5242 -> SJR-BTM331; footprint ti:PCM5242RHBR -> misc:SJR-BTM331; moved to B.Cu
- U6: value TPS54360DDA -> PCM5242; footprint Package_SO:TI_SO-PowerPAD-8_ThermalVias -> ti:PCM5242RHBR
- U8: renamed from U7; value LT3045xMSE-1 -> TPS54360DDA; footprint Package_SO:MSOP-12-1EP_3x4mm_P0.65mm_EP1.65x2.85mm -> Package_SO:TI_SO-PowerPAD-8_ThermalVias
- U9: renamed from U8; value LT3094xMSE -> LT3045xMSE-1
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- renumbered C34 to C33, C56 to C57, C57 to C58
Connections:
- C11 pad 1: +3V3 -> /stm32/NRST
- C12 pad 1: +3V3 -> /stm32/encoder_sw
- C13 pad 1: /stm32/AVDD -> /stm32/encoder_a
- C14 pad 1: /stm32/AVDD -> /stm32/encoder_b
- C15 pad 1: +3V3 -> VCC
- C16 pad 1: /stm32/NRST -> Net-(C16-Pad1)
- C17 pad 1: +3V3 -> Net-(C17-Pad1)
- C18 pad 1: VCC -> Net-(C18-Pad1)
- C18 pad 2: GND -> Net-(C18-Pad2)
- C19 pad 1: /Sheet6035C8EF/CPVDD -> VDD
- C2 pad 1: /Sheet6035C8EF/CPVDD -> +3V3
- C20 pad 1: VCC -> VDD
- C21 pad 1: Net-(C21-Pad1) -> +3V3
- C22 pad 1: Net-(C23-Pad1) -> /Bluetooth/vdd_x
- C23 pad 1: Net-(C24-Pad1) -> /Bluetooth/vdd_x
- C23 pad 2: Net-(C24-Pad2) -> GND
- C25 pad 1: +3V3 -> /Sheet6035C8EF/CPVDD
- C27 pad 1: VDD -> GND
- C27 pad 2: GND -> Net-(C27-Pad2)
- C28 pad 1: VDD -> Net-(C28-Pad1)
- C28 pad 2: GND -> Net-(C28-Pad2)
- C3 pad 1: /stm32/encoder_sw -> +3V3
- C31 pad 1: /Sheet6035C8EF/AVDD -> Net-(C31-Pad1)
- C36 pad 2: Net-(C36-Pad2) -> -15V
- C37 pad 1: +15V -> Net-(C37-Pad1)
- C4 pad 1: /stm32/encoder_a -> +3V3
- C41 pad 1: +15V -> Net-(C41-Pad1)
- C41 pad 2: GND -> Net-(C41-Pad2)
- C42 pad 1: +15V -> Net-(C42-Pad1)
- C42 pad 2: GND -> -15V
- C43 pad 1: Net-(C40-Pad1) -> +15V
- C43 pad 2: Net-(C36-Pad2) -> GND
- C44 pad 1: +15V -> GND
- C44 pad 2: GND -> -15V
- C46 pad 1: -15V -> GND
- C46 pad 2: GND -> Net-(C46-Pad2)
- C47 pad 1: -15V -> +12V
- C49 pad 1: Net-(C48-Pad1) -> +12V
- C5 pad 1: /stm32/encoder_b -> /stm32/AVDD
- C50 pad 1: GND -> +12V
- C50 pad 2: Net-(C36-Pad2) -> GND
- C51 pad 1: -15V -> Net-(C51-Pad1)
- C51 pad 2: GND -> Net-(C51-Pad2)
- C52 pad 1: Net-(C48-Pad1) -> Net-(C52-Pad1)
- C52 pad 2: GND -> Net-(C52-Pad2)
- C53 pad 1: GND -> +12V
- C53 pad 2: Net-(C36-Pad2) -> GND
- C55 pad 1: Net-(C54-Pad1) -> +12V
- C56 pad 1: GND -> -12V
- C56 pad 2: Net-(C55-Pad2) -> GND
- C57 pad 1: +15V -> -12V
- C58 pad 1: GND -> -12V
- C58 pad 2: -15V -> GND
- C59 pad 1: Net-(C59-Pad1) -> -12V
- C59 pad 2: Net-(C59-Pad2) -> GND
- C6 pad 1: /stm32/OSC_IN -> /stm32/AVDD
- C7 pad 1: /stm32/OSC_OUT -> +3V3
- C8 pad 1: +3V3 -> /stm32/OSC_IN
- D1 pad 1: Net-(C48-Pad1) -> Net-(C18-Pad1)
- D1 pad 2: Net-(D1-Pad2) -> GND
- D2 pad 1: Net-(C42-Pad1) -> VCC
- D2 pad 2: Net-(C36-Pad2) -> Net-(D2-Pad2)
- D3 pad 2: Net-(D3-Pad2) -> Net-(D2-Pad2)
- D4 pad 1: VCC -> Net-(C38-Pad2)
- D4 pad 2: Net-(D3-Pad2) -> GND
- D5 pad 1: Net-(C24-Pad1) -> Net-(C41-Pad1)
- D5 pad 2: GND -> -15V
- D6 pad 1: Net-(D6-Pad1) -> VCC
- H1 pad 1: Net-(H1-Pad1) -> (no net)
- H2 pad 1: Net-(H2-Pad1) -> (no net)
- H3 pad 1: Net-(H3-Pad1) -> (no net)
- H4 pad 1: Net-(H4-Pad1) -> (no net)
- J2 pad 1: GND -> (no net)
- J2 pad 2: /stm32/encoder_b -> Net-(J2-Pad2)
- J2 pad 3: /stm32/encoder_a -> Net-(J2-Pad3)
- J2 pad 4: /stm32/encoder_sw -> GND
- J4 pad 1: +3V3 -> GND
- J4 pad 2: +3V3 -> /stm32/SWDIO
- J4 pad 3: /stm32/JTRST -> /stm32/SWCLK
- J4 pad 4: GND -> /stm32/uart_out
- J5 pad 1: Net-(D3-Pad2) -> Net-(D2-Pad2)
- J5 pad 3: Net-(J5-Pad3) -> (no net)
- L1 pad 1: Net-(D1-Pad2) -> Net-(C18-Pad1)
- L1 pad 2: GND -> VDD
- L2 pad 1: Net-(C24-Pad1) -> +15V
- L2 pad 2: VDD -> Net-(C38-Pad2)
- R10 pad 1: /stm32/USB_CO -> +3V3
- R10 pad 2: Net-(Q1-Pad1) -> /stm32/USB_CO
- R11 pad 1: +3V3 -> /stm32/USB_CO
- R11 pad 2: /stm32/USB_CO -> Net-(Q1-Pad1)
- R12 pad 1: /stm32/AVDD -> +3V3
- R12 pad 2: +3V3 -> /stm32/encoder_sw
- R13 pad 2: /stm32/NRST -> /stm32/encoder_a
- R14 pad 1: Net-(J4-Pad17) -> +3V3
- R14 pad 2: GND -> /stm32/encoder_b
- R15 pad 1: Net-(J4-Pad19) -> VCC
- R15 pad 2: GND -> Net-(R15-Pad2)
- R16 pad 1: Net-(J4-Pad11) -> Net-(R15-Pad2)
- R17 pad 1: Net-(J3-PadA5) -> Net-(R17-Pad1)
- R18 pad 1: VCC -> Net-(C17-Pad1)
- R18 pad 2: Net-(R18-Pad2) -> Net-(C16-Pad1)
- R19 pad 1: Net-(R18-Pad2) -> VDD
- R19 pad 2: GND -> Net-(R19-Pad2)
- R2 pad 1: +3V3 -> /stm32/AVDD
- R2 pad 2: /stm32/encoder_sw -> +3V3
- R20 pad 1: Net-(R20-Pad1) -> Net-(R19-Pad2)
- R21 pad 1: Net-(C23-Pad1) -> +3V3
- R21 pad 2: Net-(C21-Pad1) -> Net-(R21-Pad2)
- R22 pad 1: +3V3 -> /Bluetooth/vdd_x
- R22 pad 2: Net-(R22-Pad2) -> +3V3
- R23 pad 1: VDD -> /Sheet6035C8EF/CPVDD
- R23 pad 2: Net-(R23-Pad2) -> +3V3
- R24 pad 1: Net-(R23-Pad2) -> /Sheet6035C8EF/AVDD
- R24 pad 2: GND -> +3V3
- R25 pad 1: +3V3 -> /Sheet6035C8EF/DVDD
- R25 pad 2: Net-(D6-Pad1) -> +3V3
- R27 pad 1: +3V3 -> Net-(R27-Pad1)
- R27 pad 2: /stm32/encoder_a -> -15V
- R29 pad 1: /Sheet6035C8EF/AVDD -> Net-(C40-Pad1)
- R29 pad 2: +3V3 -> Net-(C42-Pad1)
- R3 pad 1: +3V3 -> /stm32/OSC_OUT
- R3 pad 2: /SCL -> /stm32/OSC_IN
- R32 pad 1: /Sheet6035C8EF/CPVDD -> GND
- R32 pad 2: +3V3 -> /Sheet6035C8EF/sheet5FF87CA5/FB2
- R34 pad 1: /Sheet6035C8EF/DVDD -> Net-(R34-Pad1)
- R34 pad 2: +3V3 -> GND
- R35 pad 1: Net-(C40-Pad1) -> Net-(C45-Pad1)
- R35 pad 2: Net-(C43-Pad1) -> GND
- R36 pad 1: Net-(R31-Pad1) -> GND
- R36 pad 2: Net-(C36-Pad2) -> Net-(R36-Pad2)
- R37 pad 1: Net-(C48-Pad1) -> GND
- R37 pad 2: Net-(R33-Pad2) -> Net-(C46-Pad2)
- R38 pad 1: Net-(R33-Pad2) -> Net-(C51-Pad1)
- R38 pad 2: Net-(C36-Pad2) -> /Sheet6035C8EF/OUTLP
- R39 pad 1: Net-(R35-Pad1) -> Net-(C51-Pad2)
- R39 pad 2: GND -> /Sheet6035C8EF/OUTLN
- R4 pad 2: /SDA -> /stm32/NRST
- R40 pad 1: GND -> Net-(C52-Pad2)
- R40 pad 2: Net-(R36-Pad2) -> /Sheet6035C8EF/OUTRN
- R41 pad 1: Net-(C54-Pad1) -> Net-(C52-Pad1)
- R41 pad 2: GND -> /Sheet6035C8EF/OUTRP
- R42 pad 1: GND -> Net-(R42-Pad1)
- R42 pad 2: Net-(C55-Pad2) -> Net-(C51-Pad1)
- R43 pad 1: Net-(J3-PadA4) -> Net-(R43-Pad1)
- R43 pad 2: GND -> Net-(C51-Pad2)
- R44 pad 1: /headphone_in -> Net-(R44-Pad1)
- R44 pad 2: Net-(J7-PadSN) -> Net-(C52-Pad2)
- R47 pad 1: Net-(R47-Pad1) -> Net-(R45-Pad1)
- R47 pad 2: Net-(C58-Pad1) -> GND
- R48 pad 1: Net-(R48-Pad1) -> Net-(R43-Pad1)
- R48 pad 2: Net-(C58-Pad2) -> /Sheet6035C8EF/sheet5FF9330D/LOUT
- R49 pad 1: /Sheet6035C8EF/sheet5FF9330D/ROUT -> Net-(R44-Pad1)
- R49 pad 2: Net-(J7-PadR) -> /Sheet6035C8EF/sheet5FF9330D/ROUT
- R5 pad 1: /stm32/OSC_OUT -> +3V3
- R5 pad 2: /stm32/OSC_IN -> /SCL
- R50 pad 1: /Sheet6035C8EF/sheet5FF9330D/LOUT -> /headphone_in
- R50 pad 2: Net-(J7-PadT) -> Net-(J6-PadR2)
- R51 pad 1: Net-(R47-Pad1) -> /Sheet6035C8EF/sheet5FF9330D/ROUT
- R51 pad 2: GND -> Net-(J6-PadR1)
- R52 pad 1: Net-(R50-Pad1) -> /Sheet6035C8EF/sheet5FF9330D/LOUT
- R52 pad 2: GND -> Net-(J6-PadT)
- R53 pad 1: Net-(R48-Pad1) -> Net-(R53-Pad1)
- R53 pad 2: /Sheet6035C8EF/sheet5FF9330D/LOUT -> Net-(R53-Pad2)
- R54 pad 1: Net-(R49-Pad1) -> Net-(R53-Pad2)
- R54 pad 2: /Sheet6035C8EF/sheet5FF9330D/ROUT -> GND
- R7 pad 1: Net-(J3-PadA6) -> +3V3
- R7 pad 2: Net-(Q1-Pad3) -> /SDA
- R8 pad 2: Net-(J3-PadA6) -> Net-(J2-Pad3)
- R9 pad 2: Net-(J3-PadA7) -> Net-(J2-Pad2)
- U1 pad 1: /stm32/SPDIF_RX -> +3V3
- U1 pad 2: GND -> /headphone_in
- U1 pad 3: +3V3 -> (no net)
- U10 pad 10: GND -> -12V
- U10 pad 11: GND -> -12V
- U10 pad 12: GND -> -12V
- U10 pad 13: GND -> -15V
- U10 pad 2: /Sheet6035C8EF/sheet5FF9330D/LOUT -> -15V
- U10 pad 3: +15V -> -15V
- U10 pad 4: Net-(R47-Pad1) -> Net-(R36-Pad2)
- U10 pad 5: Net-(R48-Pad1) -> -15V
- U10 pad 7: GND -> (no net)
- U10 pad 8: GND -> Net-(C46-Pad2)
- U13 pad 1: Net-(U13-Pad1) -> Net-(R53-Pad2)
- U13 pad 2: Net-(U13-Pad2) -> Net-(R53-Pad1)
- U13 pad 3: /I2S1_SD -> /Sheet605867F7/vcc_x
- U2 pad 1: +3V3 -> /stm32/SPDIF_RX
- U2 pad 2: /headphone_in -> GND
- U2 pad 3: Net-(U2-Pad3) -> +3V3
- U3 pad 1: Net-(C24-Pad2) -> Net-(C18-Pad2)
- U3 pad 3: Net-(R18-Pad2) -> Net-(R15-Pad2)
- U3 pad 4: Net-(R20-Pad1) -> Net-(R17-Pad1)
- U3 pad 5: Net-(R23-Pad2) -> Net-(R19-Pad2)
- U3 pad 6: Net-(C23-Pad1) -> Net-(C17-Pad1)
- U3 pad 8: Net-(C24-Pad1) -> Net-(C18-Pad1)
- U4 pad 2: Net-(R22-Pad2) -> Net-(R21-Pad2)
- U5 pad 1: /Sheet6035C8EF/DVDD -> (no net)
- U5 pad 10: /Sheet6035C8EF/OUTLP -> (no net)
- U5 pad 11: /Sheet6035C8EF/OUTLN -> (no net)
- U5 pad 12: /Sheet6035C8EF/OUTRP -> (no net)
- U5 pad 13: /Sheet6035C8EF/OUTRN -> /BT_en
- U5 pad 14: /Sheet6035C8EF/AVDD -> /Bluetooth/vdd_x
- U5 pad 16: Net-(C25-Pad2) -> (no net)
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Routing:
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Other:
- net class signal: clearance 0.15 -> 0.2; trace_width 0.15 -> 0.2
- rule trace_min: 0.15 -> 0.2
- rule via_min_size: 0.6 -> 0.5

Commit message: digital-amplifier2-v3
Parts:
- C37, C40: value 1.3pf -> 220pF
- C39, C42: value 1.2nf -> 4.3nF
- R26, R27: value 121k -> 97.6kOhm
- R28, R29: value 68.1k -> 18.7kOhm
